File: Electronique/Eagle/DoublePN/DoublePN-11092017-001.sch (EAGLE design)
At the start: 127 parts, among them IC1 MC78M09CDTG, T1 MMBT2222ALT1, T2 MMBT2222ALT1, T3 MMBT2222ALT1, T4 MMBT2222ALT1

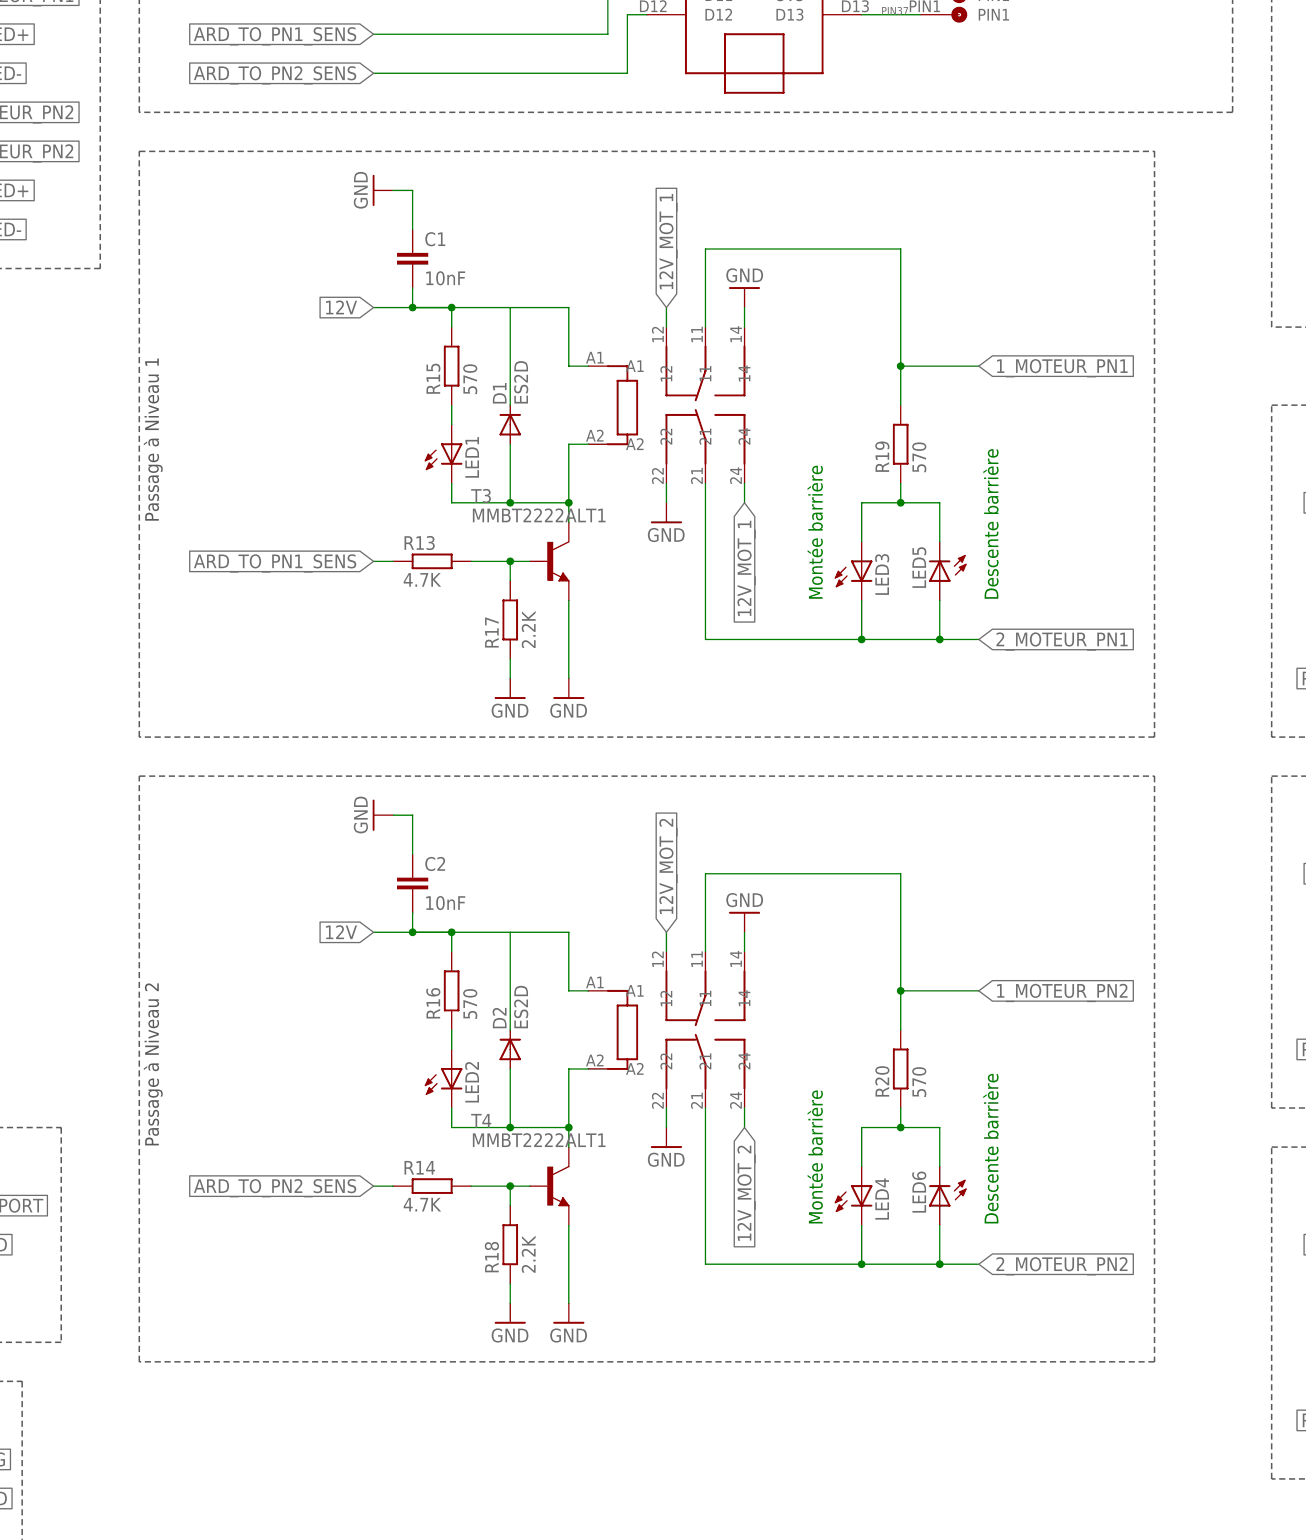
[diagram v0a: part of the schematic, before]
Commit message: Mise à jour carte
Mise à jour carte
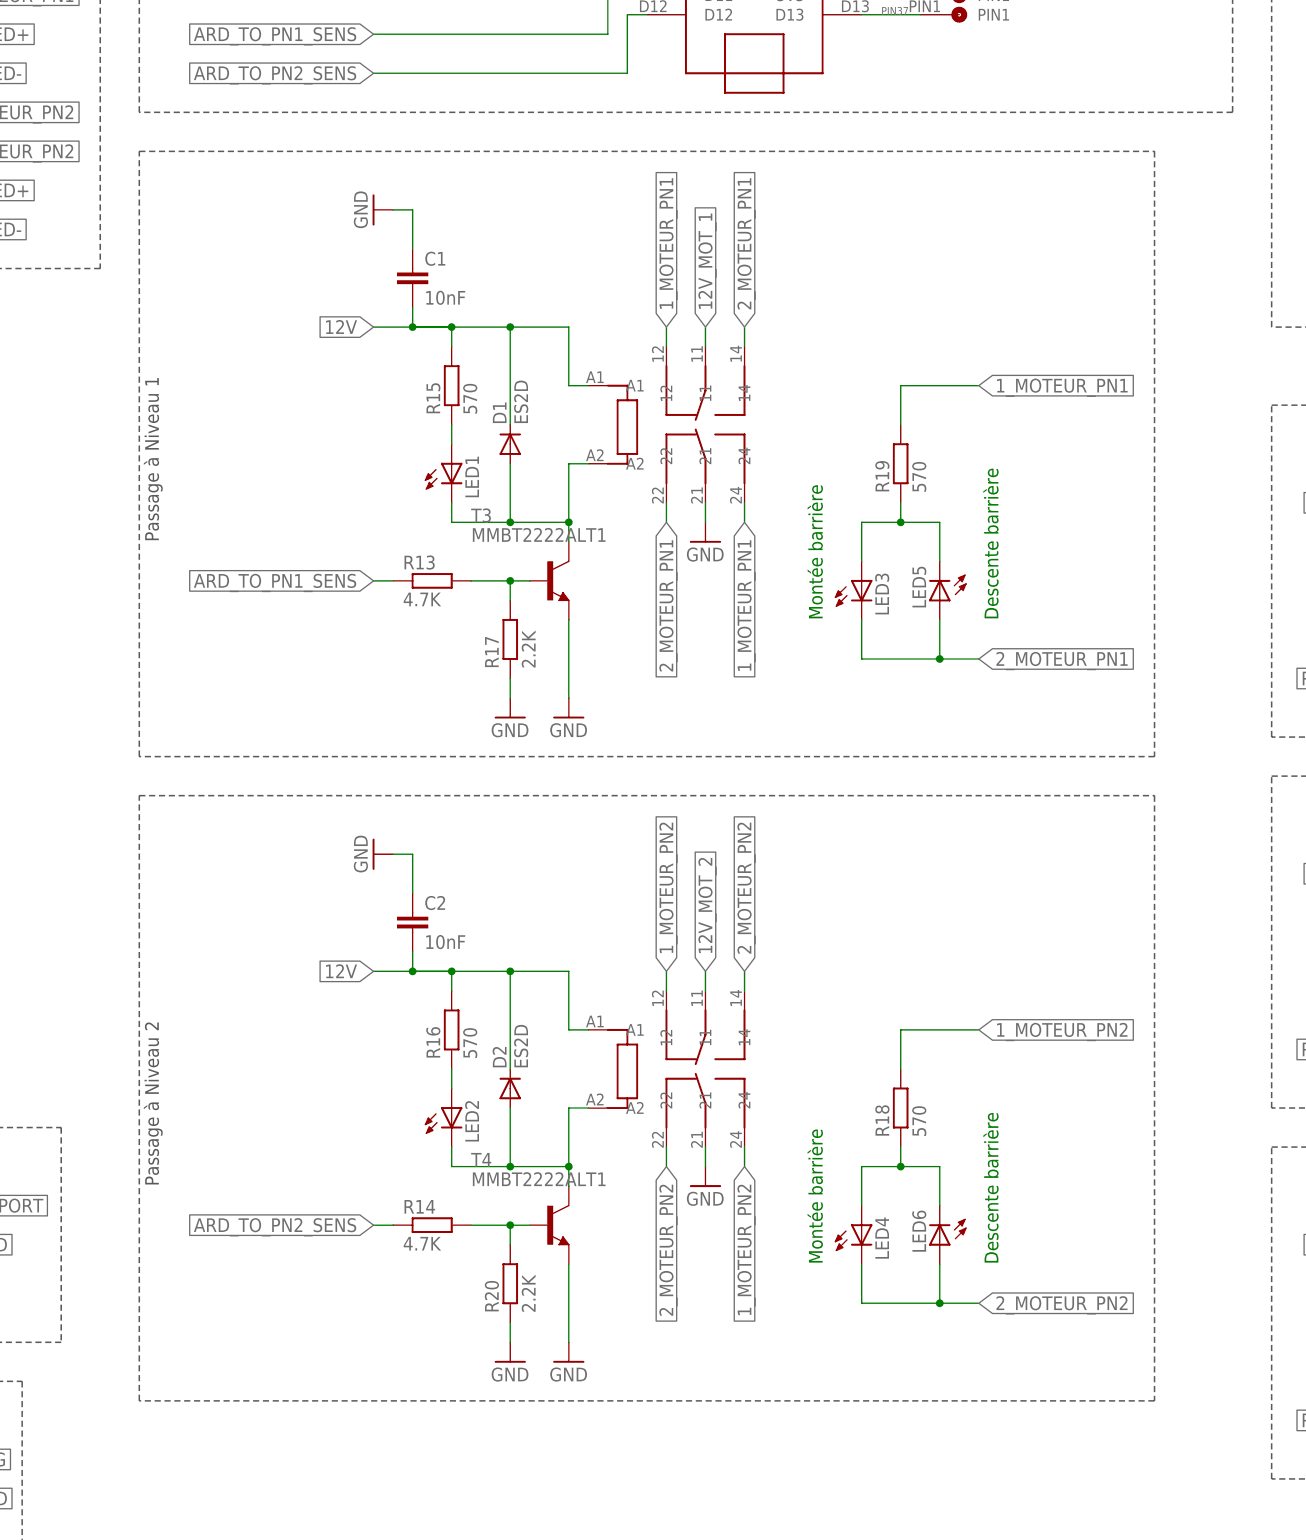
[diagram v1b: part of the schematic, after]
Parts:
- R18: value 2.2K -> 570
- R20: value 570 -> 2.2K
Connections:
- net 12V_MOT_1: now also RLS1.11; no longer RLS1.12, RLS1.24
- net 12V_MOT_2: now also RLS2.11; no longer RLS2.12, RLS2.24
- net 1_MOTEUR_PN1: now also RLS1.12, RLS1.24; no longer RLS1.11
- net 1_MOTEUR_PN2: now also R18.2, RLS2.12, RLS2.24; no longer R20.2, RLS2.11
- net 2_MOTEUR_PN1: now also RLS1.14, RLS1.22; no longer RLS1.21
- net 2_MOTEUR_PN2: now also RLS2.14, RLS2.22; no longer RLS2.21
- net FEU_PN1: now also ARDUINO-NANO1.D9
- net FEU_PN2: now also ARDUINO-NANO1.D10
- net GND: now also R20.1, RLS1.21, RLS2.21; no longer R18.1, RLS1.14, RLS1.22, RLS2.14, RLS2.22
- net N$16: now also R18.1; no longer R20.1
- net N$17: now also R20.2; no longer R18.2
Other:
- moved on the sheet: C1, C2, D1, D2, LED1, LED2, LED3, LED4, LED5, LED6, R13, R14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
